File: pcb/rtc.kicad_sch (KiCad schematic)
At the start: 2 parts, among them U3 SW_Push

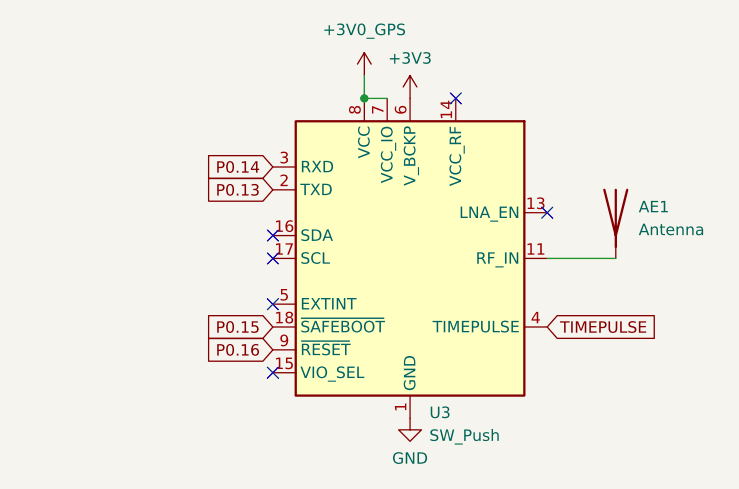
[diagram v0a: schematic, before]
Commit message: sus commit
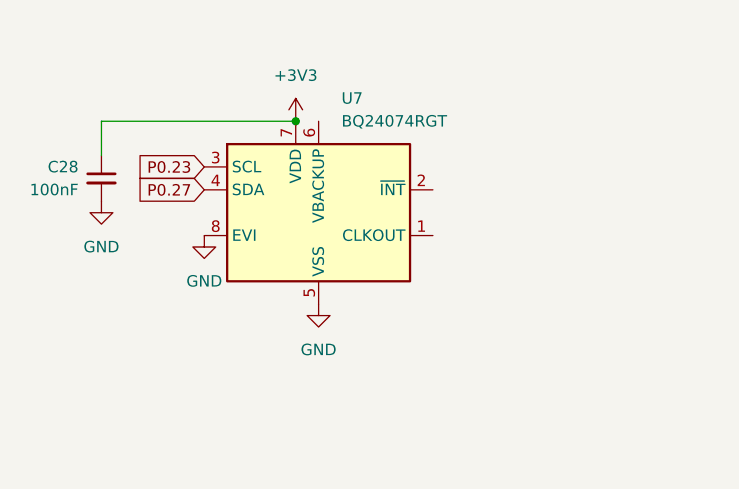
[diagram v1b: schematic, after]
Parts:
- removed AE1: Antenna, JLCImport:KH-GPS181804-WY, symbol Device:Antenna
- removed U3: SW_Push, symbol RF_GPS:MAX-M10S
- added C28: 100nF, Capacitor_SMD:C_0402_1005Metric, symbol Device:C_Small
- added U7: BQ24074RGT, Package_DFN_QFN:VQFN-16-1EP_3x3mm_P0.5mm_EP1.6x1.6mm, symbol Timer_RTC:RV-3028-C7
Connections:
- net +3V3: now also C28.1, U7.7 (VDD)
- net GND: now also C28.2, U7.5 (VSS), U7.8 (EVI)
- new net P0.23: U7.3 (SCL)
- new net P0.27: U7.4 (SDA)
- no-connect marks 6 -> 0
